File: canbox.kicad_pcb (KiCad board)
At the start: 2 copper layers, 80 x 50 mm, 108 parts, among them J1 Conn_ARM_SWD_NXP, J2 Screw_Terminal_01x02, J3 Screw_Terminal_01x02, J4 Conn_ARM_JTAG_SWD_20, J5 DB9_Male, J7 USB_B_Micro, K2 FTR-K3AB005W, U1 LPC54616J512, U11 MP1582, U3 TJA1102SHN, U5 TJA1051T, U6 TLV70233_SOT23-5, U7 KeyMatrix, U8 ULN2003ADRG3, Y1 12MHz, Y2 32.768k, Y3 25Mhz

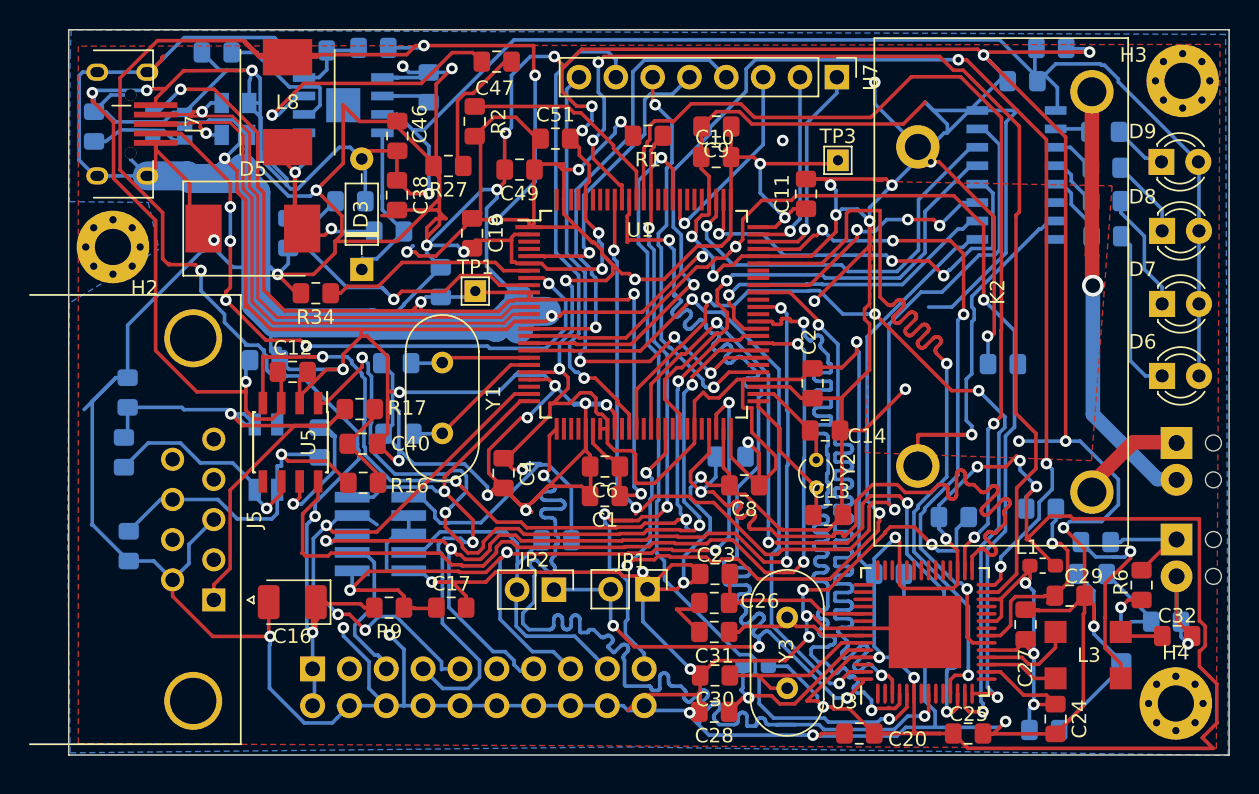
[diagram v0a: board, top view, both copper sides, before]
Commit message: Fix few bugs, review design
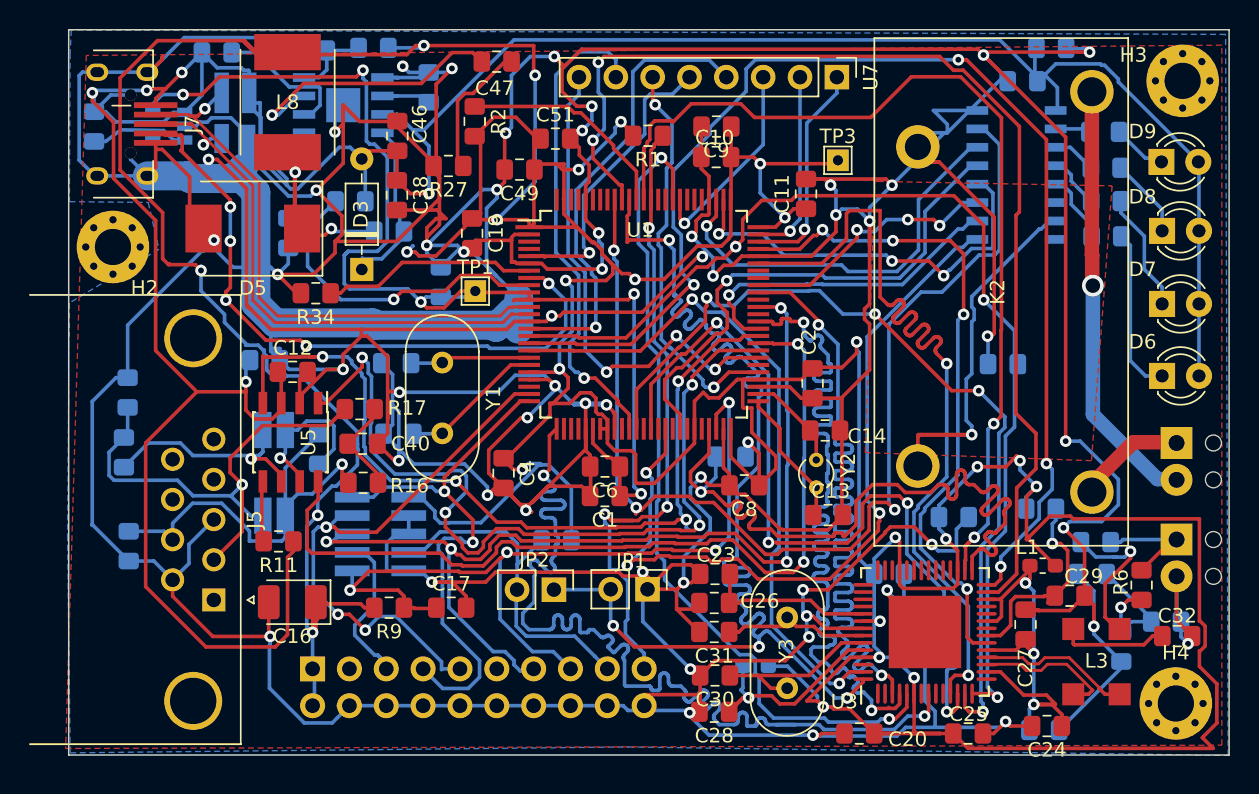
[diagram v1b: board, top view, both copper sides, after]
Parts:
- added R11: NC, Resistor_SMD:R_0805_2012Metric_Pad1.15x1.40mm_HandSolder, F.Cu at (49.5, 117.3)
- D1: footprint Package_TO_SOT_SMD:SOT-143 -> Package_TO_SOT_SMD:SOT-143_Handsoldering
- moved L5 1.22 mm to (49.2, 112.5)
- moved C24 0.76 mm to (102.4, 130.0), turned to 180 degrees
- moved L3 0.73 mm to (105.9, 125.6), turned to 90 degrees
- moved R12 0.45 mm to (52.3, 110.9), turned to 90 degrees
- turned D5 to 180 degrees
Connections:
- D5 pad 1: GND -> Net-(C45-Pad1)
- D5 pad 2: Net-(C45-Pad1) -> GND
- J5 pad 1: /CAN/CAN_L -> (no net)
- J5 pad 2: (no net) -> /CAN/CAN_L
- J5 pad 7: (no net) -> /CAN/CAN_H
- J5 pad 8: /CAN/CAN_H -> (no net)
- L5 pad 3: /CAN/CAN_L -> Net-(L5-Pad3)
- L5 pad 4: Net-(L5-Pad4) -> /CAN/CAN_L
- R13 pad 1: Net-(L5-Pad4) -> Net-(L5-Pad3)
- U3 pad 17: /Ethernet/TRX_0_T_N -> /Ethernet/TRX_0_T_P
- U3 pad 18: /Ethernet/TRX_0_T_P -> /Ethernet/TRX_0_T_N
- U3 pad 48: (no net) -> +3V3
- U5 pad 5: (no net) -> Net-(R11-Pad2)
- U5 pad 6: Net-(L5-Pad4) -> Net-(L5-Pad3)
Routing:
- net GND: track 949.1 -> 879.2 mm, vias 59 -> 53
- net 5V: track 192.2 -> 221.6 mm
- net Net-(L5-Pad3): track 0.00 -> 16.7 mm, vias 0 -> 1
- net Net-(L5-Pad4): track 15.6 -> 0.00 mm, vias 1 -> 0
- net /Ethernet/TRX_0_T_N: track 5.14 -> 11.4 mm
- net /CAN/CAN_H: track 24.4 -> 29.6 mm
- net /MCU/3V3_LC: track 77.8 -> 82.6 mm, vias 4 -> 5
- net /Ethernet/TRX_0_P: track 2.98 -> 7.43 mm
- net Net-(R11-Pad2): track 0.00 -> 4.22 mm
- net /Ethernet/TRX_0_T_P: track 6.50 -> 9.89 mm
- net /PowerSupply/D+: track 41.3 -> 38.1 mm
- net /CAN/CAN_L: track 40.3 -> 37.2 mm
- net Net-(C22-Pad1): track 30.2 -> 33.2 mm
- net /Ethernet/TRX_0_N: track 14.1 -> 11.2 mm
- net Net-(L5-Pad2): track 14.1 -> 11.2 mm
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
